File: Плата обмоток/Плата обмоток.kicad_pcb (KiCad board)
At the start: 4 copper layers, 58 x 58 mm, 22 parts, among them J1 4900, J10 4900, J11 4900, J12 4900, J13 4900, J14 Conn_01x02, J15 C1, J16 Conn_01x02, J17 A2, J18 B1, J19 Conn_01x02, J2 4900, J3 4900, J4 Conn_02x02_Odd_Even, J5 C2, J6 A1, J7 B2, J8 4900, J9 4900

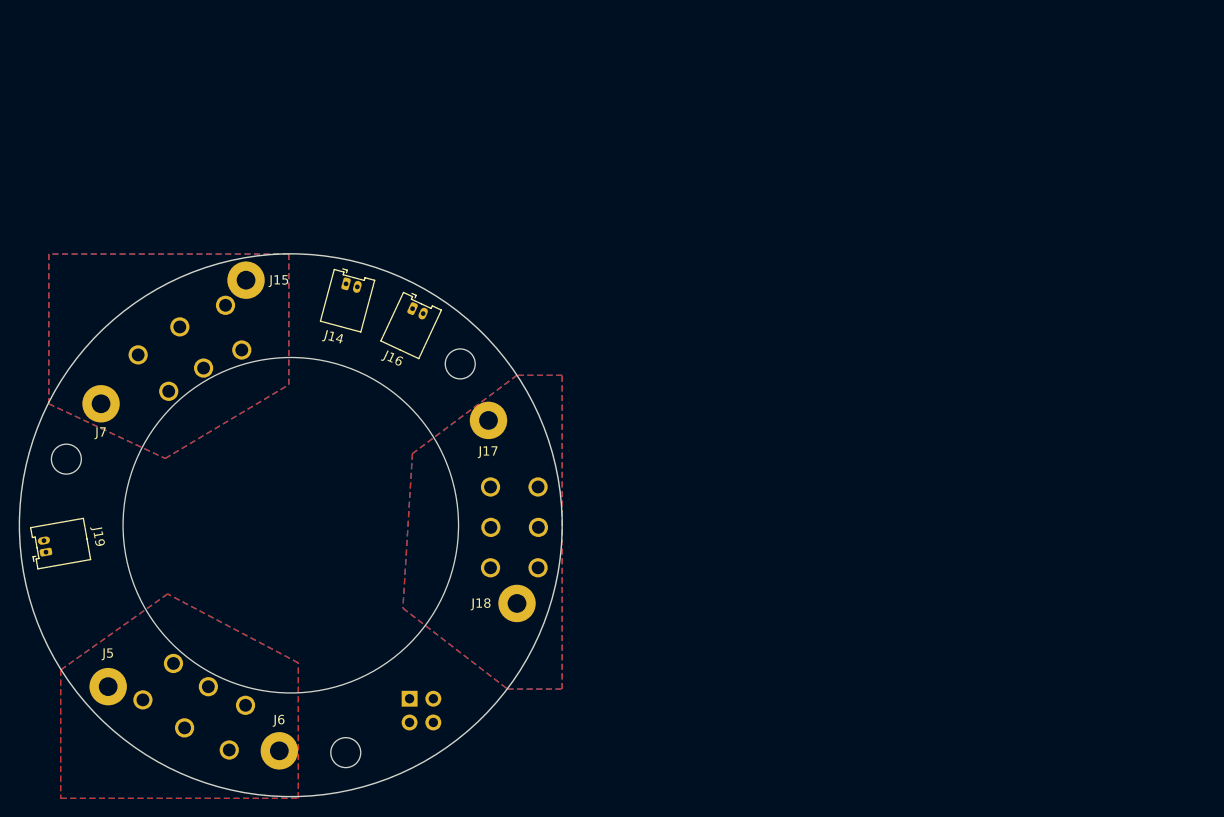
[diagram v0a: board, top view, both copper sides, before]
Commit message: VER2.0
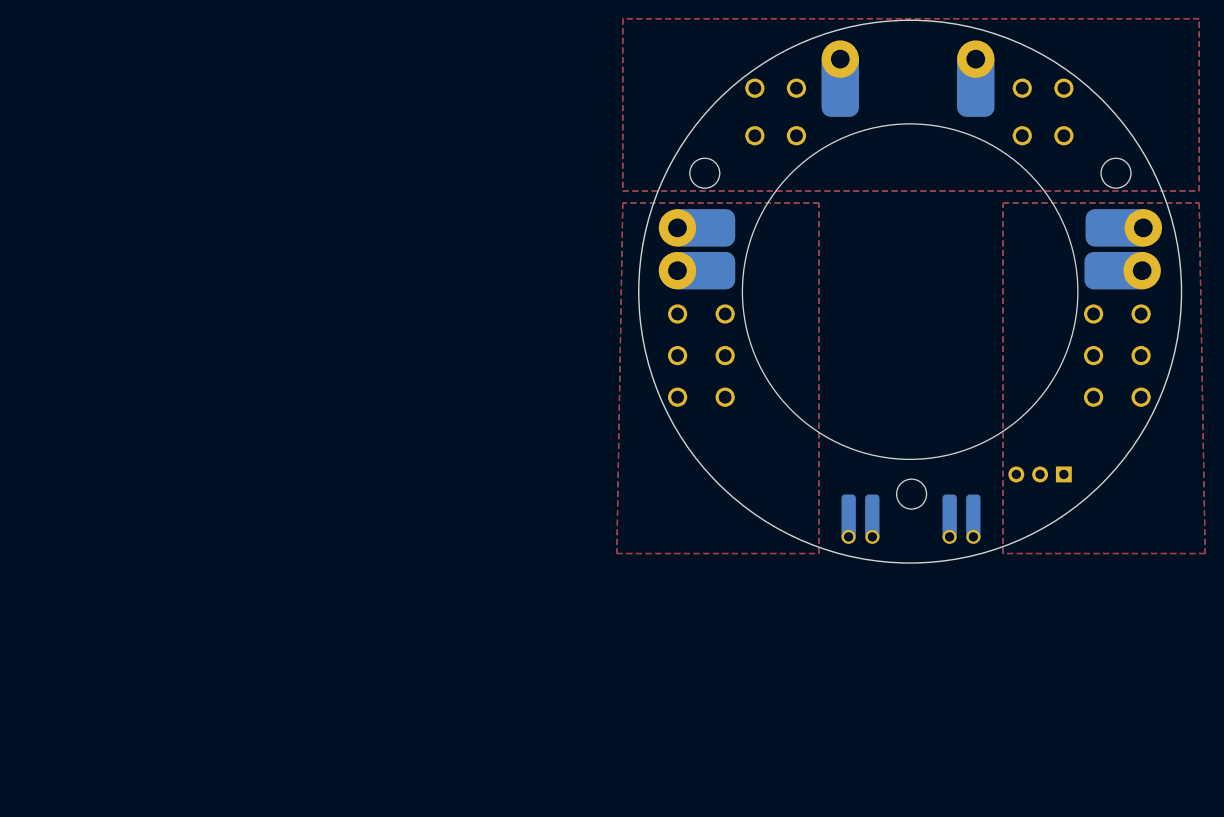
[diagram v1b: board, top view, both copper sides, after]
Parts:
- added J20: B1, Connector_My:temp_wire, B.Cu at (156.2, 97.3)
- added J21: B1, Connector_My:temp_wire, B.Cu at (145.4, 97.3)
- J14: value Conn_01x02 -> Conn_01x03; footprint Connector_Molex:Molex_PicoBlade_53048-0210_1x02_P1.25mm_Horizontal -> Connector_PinSocket_2.54mm:PinSocket_1x03_P2.54mm_Vertical; moved to B.Cu
- J15, J17, J18, J5, J6, J7: moved to B.Cu
- J16: value Conn_01x02 -> 4900; footprint Connector_Molex:Molex_PicoBlade_53048-0210_1x02_P1.25mm_Horizontal -> Connector_My:3551; moved to B.Cu
- J19: value Conn_01x02 -> B1; footprint Connector_Molex:Molex_PicoBlade_53048-0210_1x02_P1.25mm_Horizontal -> Connector_My:temp_wire; moved to B.Cu
- J4: value Conn_02x02_Odd_Even -> B1; footprint Connector_PinSocket_2.54mm:PinSocket_2x02_P2.54mm_Vertical -> Connector_My:temp_wire
- moved H2 116.3 mm to (171.4, 58.4)
- moved J3 101.7 mm to (165.9, 54.4), turned to 90 degrees
- moved J7 100.5 mm to (156.5, 46.2), turned to 180 degrees
- moved J10 92.3 mm to (161.4, 54.4), turned to 90 degrees
- moved J19 85.8 mm to (142.9, 97.3), turned to 0 degrees
- moved J14 79.4 mm to (165.9, 90.6), turned to 90 degrees
- moved J5 78.1 mm to (124.6, 64.3), turned to -90 degrees
- moved J18 78.0 mm to (174.4, 64.3), turned to 90 degrees
- moved J8 71.9 mm to (174.1, 77.9), turned to 180 degrees
- moved J17 71.7 mm to (174.2, 68.8), turned to 90 degrees
- moved J12 70.5 mm to (124.6, 73.5), turned to 0 degrees
- moved J15 67.8 mm to (142.0, 46.2), turned to 180 degrees
- moved J11 67.0 mm to (174.1, 73.5)
- moved J1 67.0 mm to (174.1, 82.4)
- moved J6 66.7 mm to (124.6, 68.8), turned to -90 degrees
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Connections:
- net A_OUT renamed A
- net C_OUT renamed C
- J10 pad 1: B_OUT -> B
- J10 pad 2: B_OUT -> B
- J13 pad 1: B_OUT -> B
- J13 pad 2: B_OUT -> B
- J14 pad 2: GNDA -> PTC_Coil_B
- J15 pad 1: B_OUT -> B
- J16 pad 1: PTC_Coil_B -> B
- J16 pad 2: GNDA -> B
- J19 pad 1: PTC_Coil_C -> PTC_Coil_B
- J3 pad 1: B_OUT -> B
- J3 pad 2: B_OUT -> B
- J7 pad 1: B_OUT -> B
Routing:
- net PTC_Coil_C: track 49.9 -> 0.00 mm
- net PTC_Coil_A: track 52.2 -> 15.0 mm
- net PTC_Coil_B: track 48.8 -> 25.0 mm
- added copper zone on In1.Cu, net A
- added copper zone on In2.Cu, net A
- added copper zone on B.Cu, net B
- added copper zone on F.Cu, net B
- added copper zone on In1.Cu, net B
- added copper zone on In2.Cu, net B
- added copper zone on In1.Cu, net C
- added copper zone on In2.Cu, net C
- removed copper zone on B.Cu, net B_OUT
- removed copper zone on F.Cu, net B_OUT
